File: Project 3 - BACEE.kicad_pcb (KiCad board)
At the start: 2 copper layers, 40.4 x 29.7 mm, 17 parts, among them J1 Digital pins, J2 Serial, J3 ICSP, J4 I2C, U1 DS1337S, U2 24LC1025, U3 24LC1025, U4 ATMEGA328P-AU, Y1 Crystal 32 MHz, Y2 Crystal 16 MHz

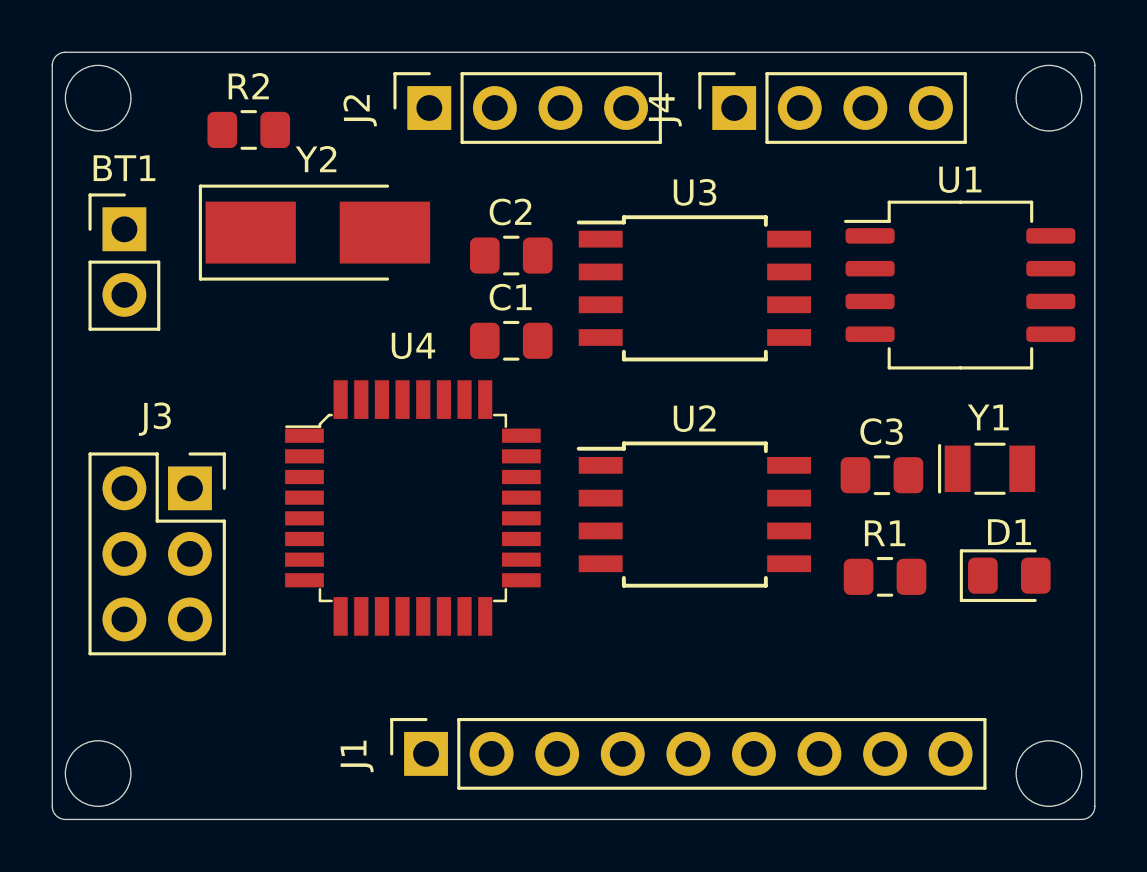
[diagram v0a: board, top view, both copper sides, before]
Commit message: Added the gerber files.
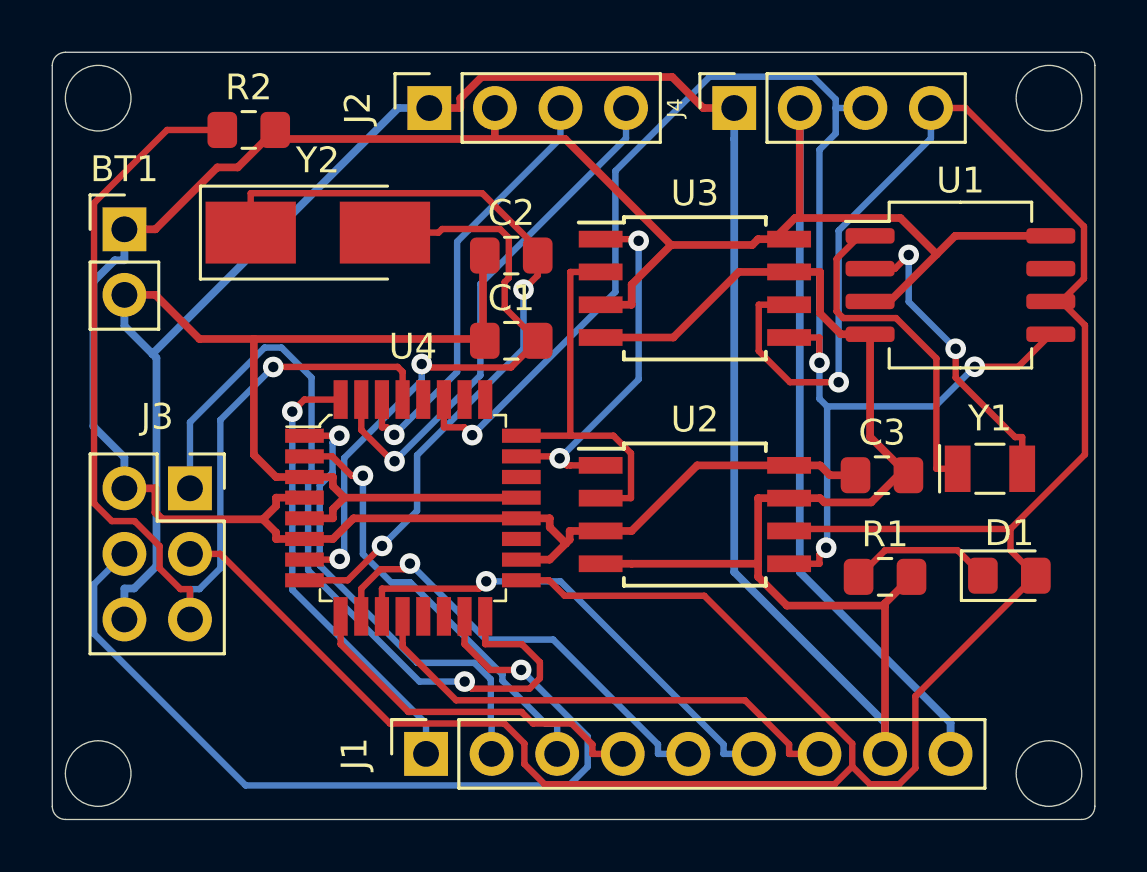
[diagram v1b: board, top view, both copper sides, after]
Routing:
- net GNDPWR: track 0.00 -> 152.3 mm
- net /VCC: track 0.00 -> 129.4 mm
- net /SCK: track 0.00 -> 110.2 mm, vias 0 -> 1
- net /SDA: track 0.00 -> 58.0 mm, vias 0 -> 4
- net /RESET: track 0.00 -> 42.0 mm, vias 0 -> 1
- net /MOSI: track 0.00 -> 33.9 mm, vias 0 -> 1
- net /MISO: track 0.00 -> 31.6 mm, vias 0 -> 1
- net Net-(C2-Pad2): track 0.00 -> 31.1 mm, vias 0 -> 2
- net Net-(C1-Pad2): track 0.00 -> 24.8 mm, vias 0 -> 2
- net /TX: track 0.00 -> 20.4 mm, vias 0 -> 1
- net /D8: track 0.00 -> 19.3 mm
- net /D7: track 0.00 -> 18.6 mm, vias 0 -> 1
- net /D3: track 0.00 -> 18.0 mm, vias 0 -> 1
- net /D2: track 0.00 -> 17.5 mm, vias 0 -> 1
- net /D6: track 0.00 -> 17.4 mm, vias 0 -> 1
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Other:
- copper layers 2 -> 4
